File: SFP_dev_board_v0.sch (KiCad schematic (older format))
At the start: 51 parts, among them J1 Conn_02x01_Row_Letter_First, J2 Conn_02x01_Row_Letter_First, P1 CONN_02X10, P2 SFP CAGE, SW1 SW_Push_Dual, SW2 SW_Push_Dual, SW3 SW_Push_Dual, SW4 SW_Push_Dual, U1 LD1117AV33, U2 SN65EPT22, U3 SN65LVELT23

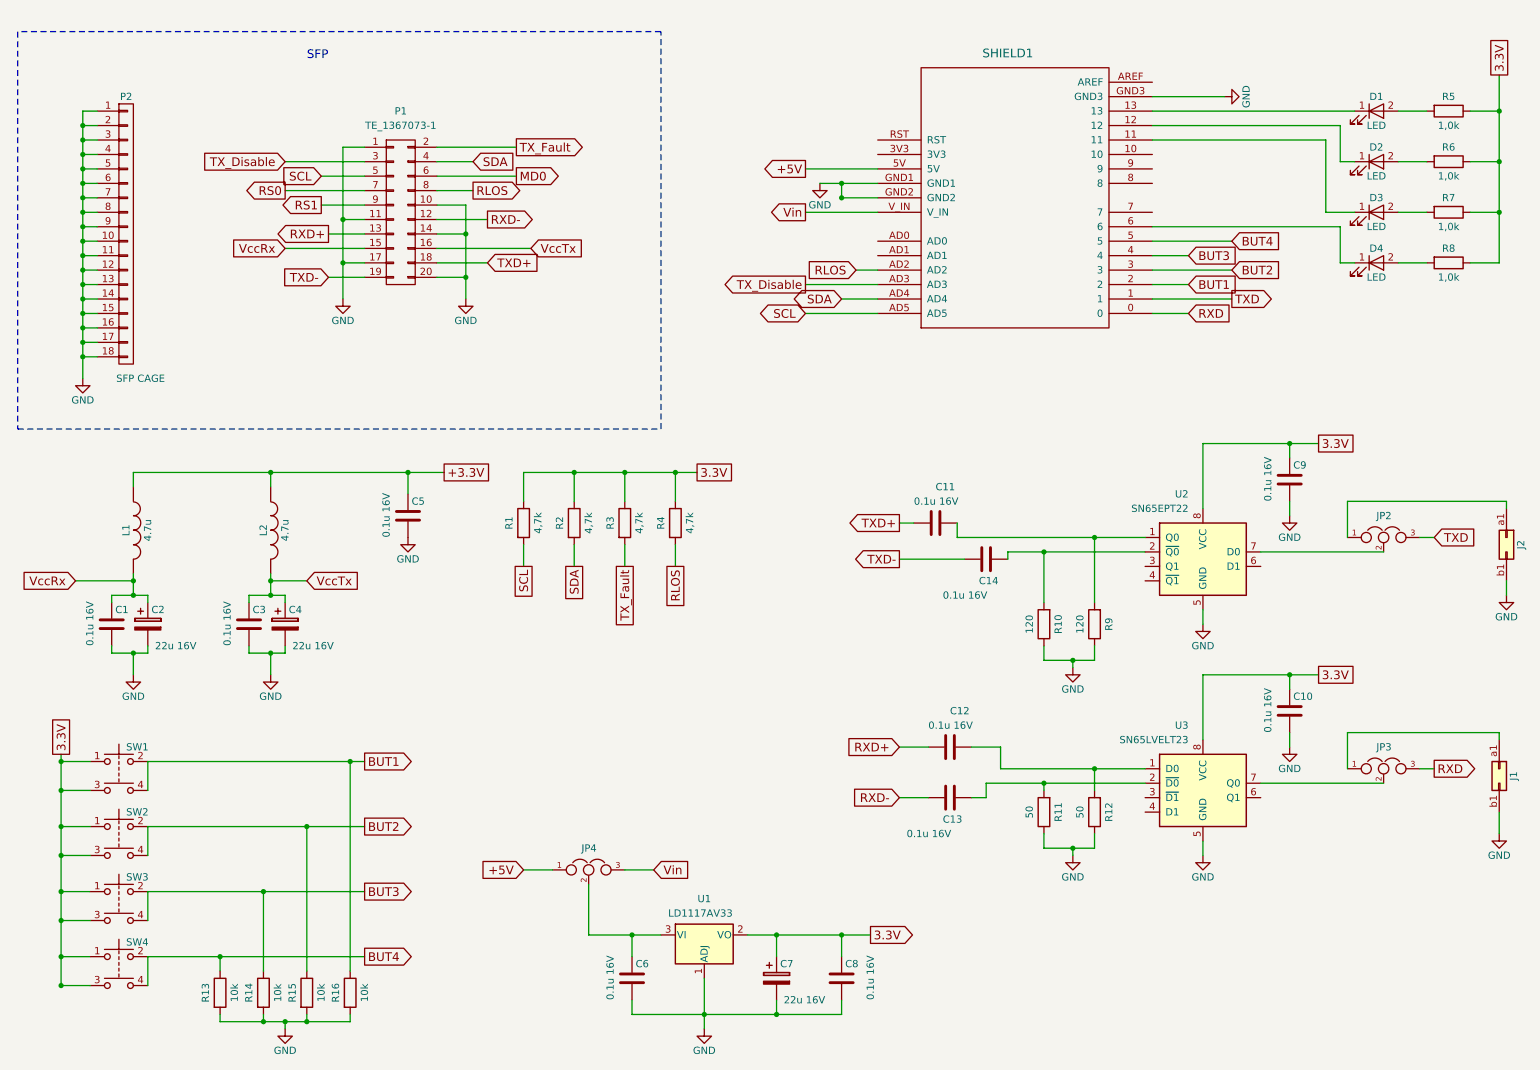
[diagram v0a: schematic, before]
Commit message: buffers
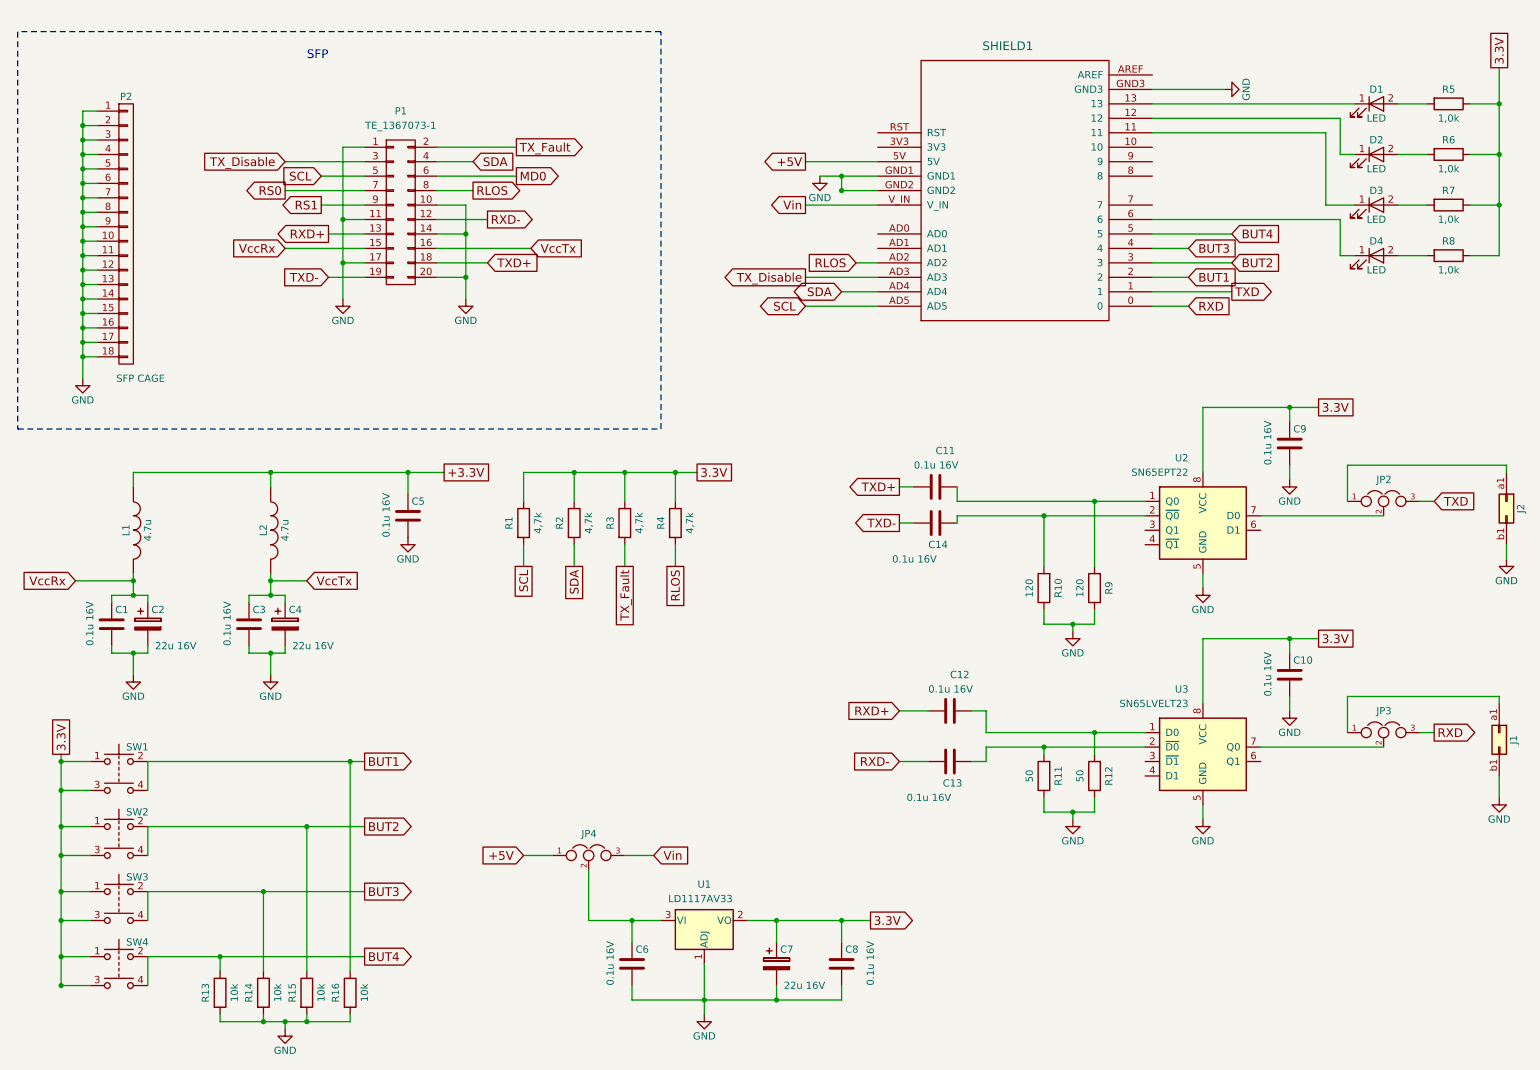
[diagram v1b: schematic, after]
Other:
- moved on the sheet: C10, C11, C12, C13, C14, C6, C7, C8, C9, D1, D2, D3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
